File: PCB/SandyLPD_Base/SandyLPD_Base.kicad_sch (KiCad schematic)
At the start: 234 parts, among them J1 Conn_02x02_Odd_Even, J10 Conn_01x10_Pin, J11 Conn_01x03, J12 Conn_01x01_Pin, J2 Conn_01x03, J3 Conn_01x01_Pin, J4 Conn_01x10_Pin, J5 USB_C_Receptacle_USB2.0, J6 USB_C_Receptacle_USB2.0, J7 USB_C_Receptacle_USB2.0, J8 USB_C_Receptacle_USB2.0, J9 Conn_02x02_Odd_Even, SW1 BOOT_ALT, SW2 RESET_ALT, SW3 SW_DIP_x04, SW4 BOOT_ALT, SW5 RESET_ALT, SW6 SW_DIP_x04, U1 NCP1117-3.3_SOT223, U2 NCP1117-3.3_SOT223, U3 RP2040, U4 W25Q128JVPIQ, U5 RP2040, U6 W25Q128JVPIQ, Y1 12MHz, Y2 12MHz

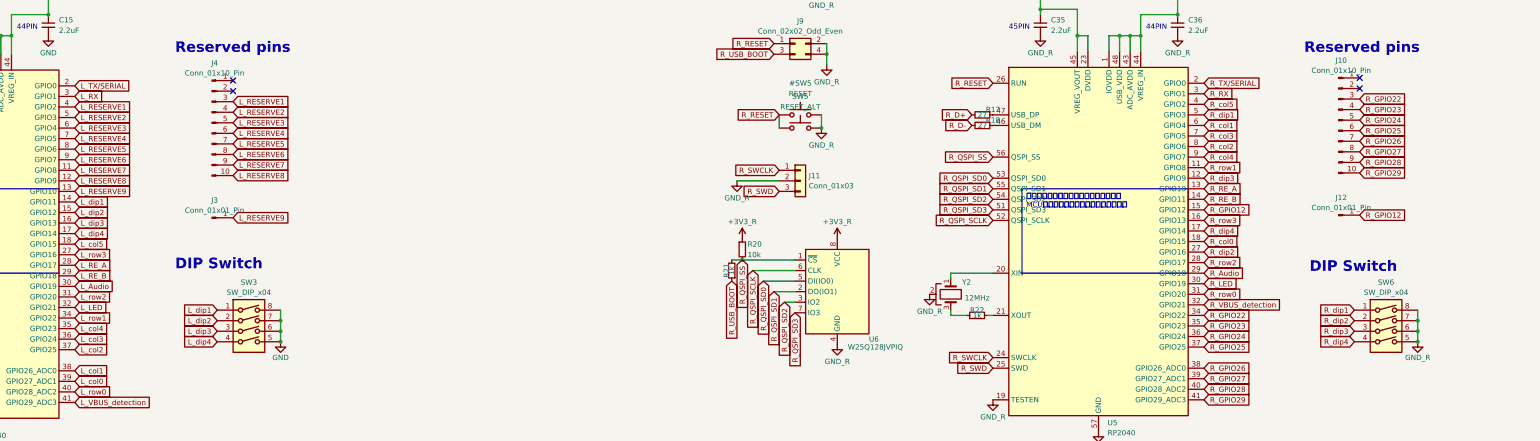
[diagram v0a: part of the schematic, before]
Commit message: 仮配線中
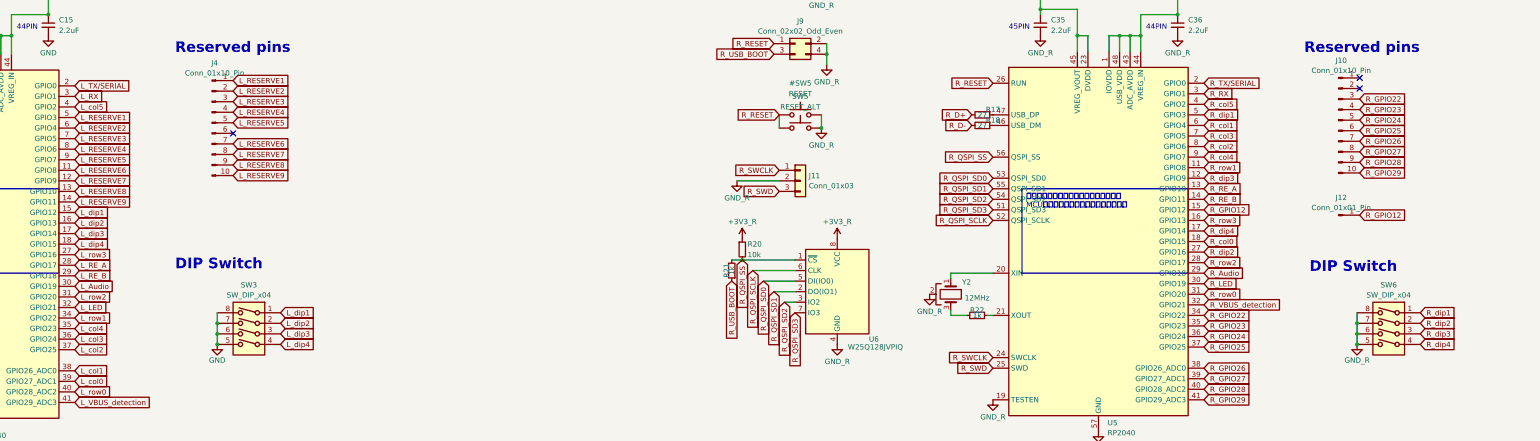
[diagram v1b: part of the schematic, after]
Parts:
- removed J3: Conn_01x01_Pin, TestPoint:TestPoint_THTPad_D1.0mm_Drill0.5mm, symbol Connector:Conn_01x01_Pin
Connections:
- net L_RESERVE1: now also J4.1 (Pin_1), U3.5 (GPIO3); no longer J4.3 (Pin_3), U3.4 (GPIO2)
- net L_RESERVE2: now also J4.2 (Pin_2), U3.6 (GPIO4); no longer J4.4 (Pin_4), U3.5 (GPIO3)
- net L_RESERVE3: now also J4.3 (Pin_3), U3.7 (GPIO5); no longer J4.5 (Pin_5), U3.6 (GPIO4)
- net L_RESERVE4: now also J4.4 (Pin_4), U3.8 (GPIO6); no longer J4.6 (Pin_6), U3.7 (GPIO5)
- net L_RESERVE5: now also J4.5 (Pin_5), U3.9 (GPIO7); no longer J4.7 (Pin_7), U3.8 (GPIO6)
- net L_RESERVE6: now also J4.7 (Pin_7), U3.11 (GPIO8); no longer J4.8 (Pin_8), U3.9 (GPIO7)
- net L_RESERVE7: now also J4.8 (Pin_8), U3.12 (GPIO9); no longer J4.9 (Pin_9), U3.11 (GPIO8)
- net L_RESERVE8: now also J4.9 (Pin_9), U3.13 (GPIO10); no longer J4.10 (Pin_10), U3.12 (GPIO9)
- net L_RESERVE9: now also J4.10 (Pin_10), U3.14 (GPIO11); no longer U3.13 (GPIO10)
- net L_col5: now also U3.4 (GPIO2); no longer U3.18 (GPIO15)
- net L_dip1: now also U3.15 (GPIO12); no longer U3.14 (GPIO11)
- net L_dip2: now also U3.16 (GPIO13); no longer U3.15 (GPIO12)
- net L_dip3: now also U3.17 (GPIO14); no longer U3.16 (GPIO13)
- net L_dip4: now also U3.18 (GPIO15); no longer U3.17 (GPIO14)
- no-connect marks 30 -> 29
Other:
- moved on the sheet: SW3, SW6
